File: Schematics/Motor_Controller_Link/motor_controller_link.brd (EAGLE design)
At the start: 160 x 100 mm, 41 parts, among them Q1 16MHz, Q2 16MHz, Q3 16MHz, U2 MC7805BDD, U3 MX150_8_PIN

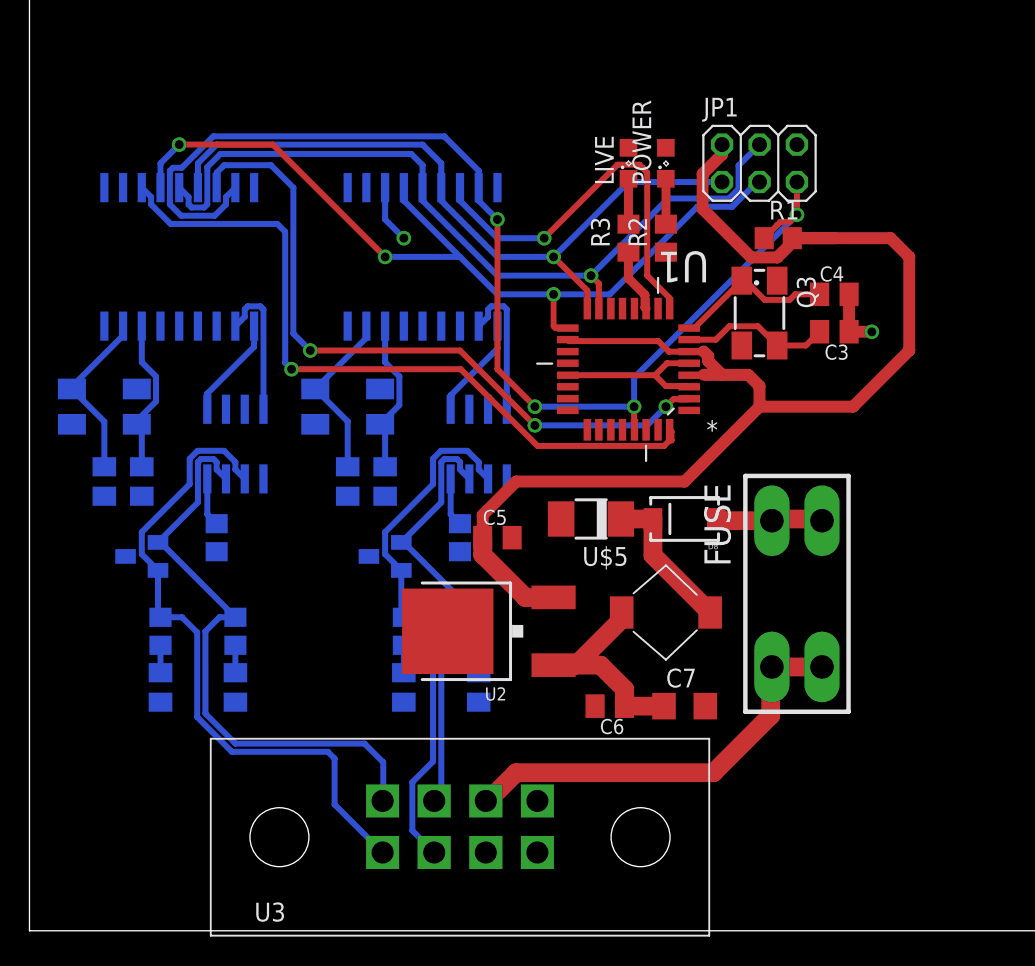
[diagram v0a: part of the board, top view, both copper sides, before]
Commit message: Figuring out power circuit
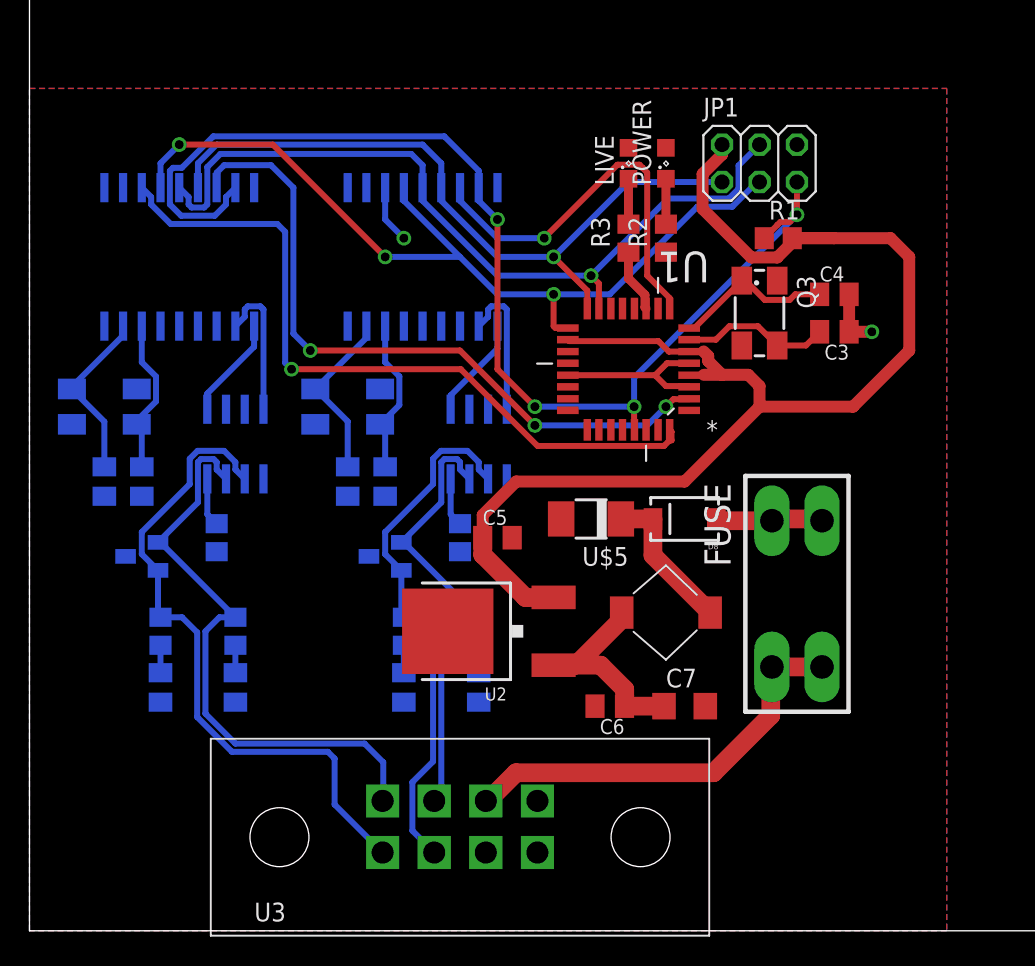
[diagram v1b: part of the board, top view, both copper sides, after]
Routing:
- added copper zone on layer 1, net GND
- added copper zone on layer 16, net GND
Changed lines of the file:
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@@
 <wire x1="8.89" y1="15.51" x2="6.52" y2="25.4" width="0" layer="19" extent="16-16"/>
 <wire x1="13.97" y1="15.51" x2="8.89" y2="15.51" width="0" layer="19" extent="16-16"/>
+<polygon width="0.4064" layer="16" isolate="0.635">
+<vertex x="0" y="57.15"/>
+<vertex x="62.23" y="57.15"/>
+<vertex x="62.23" y="0"/>
+<vertex x="0" y="0"/>
+</polygon>
+<polygon width="0.4064" layer="1" isolate="0.635">
+<vertex x="0" y="57.15"/>
+<vertex x="62.23" y="57.15"/>
+<vertex x="62.23" y="0"/>
+<vertex x="0" y="0"/>
+</polygon>
 </signal>
 <signal name="N$10">
